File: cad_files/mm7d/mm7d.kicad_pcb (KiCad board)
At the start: 2 copper layers, 56.9 x 67.6 mm, 4 parts

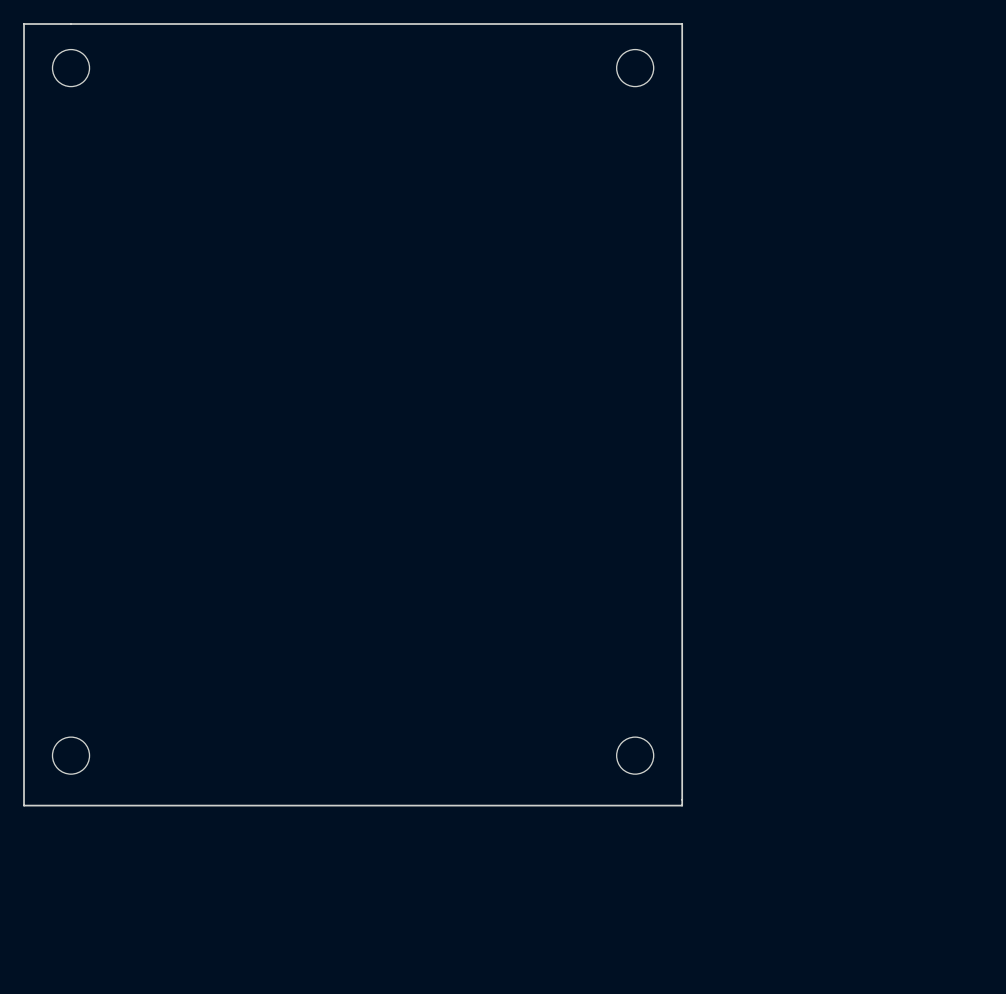
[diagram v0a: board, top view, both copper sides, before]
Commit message: 200705
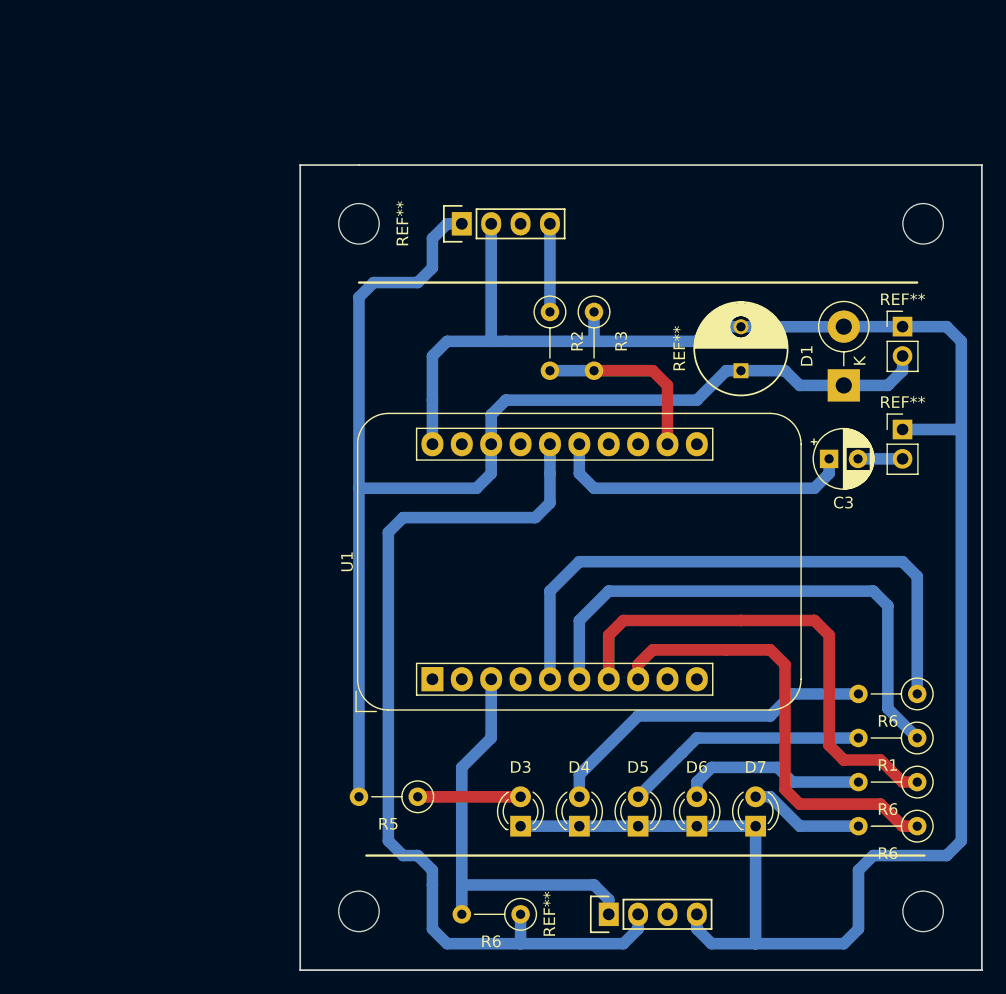
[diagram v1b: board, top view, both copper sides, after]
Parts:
- removed the REF** at (99.1, 114.0)
- removed the REF** at (147.8, 114.0)
- removed the REF** at (147.8, 54.6)
- removed the REF** at (99.1, 54.6)
- added C3: CP_Radial_D5.0mm_P2.50mm, Capacitor_THT:CP_Radial_D5.0mm_P2.50mm, F.Cu at (164.6, 88.4)
- added D1: D_5W_P5.08mm_Vertical_KathodeUp, Diode_THT:D_5W_P5.08mm_Vertical_KathodeUp, F.Cu at (165.9, 82.0)
- added D3: LED_D3.0mm, LED_THT:LED_D3.0mm, F.Cu at (137.9, 120.1)
- added D4: LED_D3.0mm, LED_THT:LED_D3.0mm, F.Cu at (143.0, 120.1)
- added D5: LED_D3.0mm, LED_THT:LED_D3.0mm, F.Cu at (148.1, 120.1)
- added D6: LED_D3.0mm, LED_THT:LED_D3.0mm, F.Cu at (153.2, 120.1)
- added D7: LED_D3.0mm, LED_THT:LED_D3.0mm, F.Cu at (158.2, 120.1)
- added R1: R_Axial_DIN0207_L6.3mm_D2.5mm_P5.08mm_Vertical, Resistor_THT:R_Axial_DIN0207_L6.3mm_D2.5mm_P5.08mm_Vertical, F.Cu at (172.2, 112.5)
- added R2: R_Axial_DIN0207_L6.3mm_D2.5mm_P5.08mm_Vertical, Resistor_THT:R_Axial_DIN0207_L6.3mm_D2.5mm_P5.08mm_Vertical, F.Cu at (140.5, 75.7)
- added R3: R_Axial_DIN0207_L6.3mm_D2.5mm_P5.08mm_Vertical, Resistor_THT:R_Axial_DIN0207_L6.3mm_D2.5mm_P5.08mm_Vertical, F.Cu at (144.3, 75.7)
- added R5: R_Axial_DIN0207_L6.3mm_D2.5mm_P5.08mm_Vertical, Resistor_THT:R_Axial_DIN0207_L6.3mm_D2.5mm_P5.08mm_Vertical, F.Cu at (129.0, 117.6)
- added R6: R_Axial_DIN0207_L6.3mm_D2.5mm_P5.08mm_Vertical, Resistor_THT:R_Axial_DIN0207_L6.3mm_D2.5mm_P5.08mm_Vertical, F.Cu at (137.9, 127.8)
- added R6: R_Axial_DIN0207_L6.3mm_D2.5mm_P5.08mm_Vertical, Resistor_THT:R_Axial_DIN0207_L6.3mm_D2.5mm_P5.08mm_Vertical, F.Cu at (172.2, 120.1)
- added R6: R_Axial_DIN0207_L6.3mm_D2.5mm_P5.08mm_Vertical, Resistor_THT:R_Axial_DIN0207_L6.3mm_D2.5mm_P5.08mm_Vertical, F.Cu at (172.2, 116.3)
- added R6: R_Axial_DIN0207_L6.3mm_D2.5mm_P5.08mm_Vertical, Resistor_THT:R_Axial_DIN0207_L6.3mm_D2.5mm_P5.08mm_Vertical, F.Cu at (172.2, 108.7)
- added REF**: PinHeader_1x02_P2.54mm_Vertical, Connector_PinHeader_2.54mm:PinHeader_1x02_P2.54mm_Vertical, F.Cu at (170.9, 77.0)
- added REF**: MountingHole_3.5mm, MountingHole:MountingHole_3.5mm, F.Cu at (172.7, 68.1)
- added REF**: MountingHole_3.5mm, MountingHole:MountingHole_3.5mm, F.Cu at (172.7, 127.5)
- added REF**: MountingHole_3.5mm, MountingHole:MountingHole_3.5mm, F.Cu at (124.0, 127.5)
- added REF**: MountingHole_3.5mm, MountingHole:MountingHole_3.5mm, F.Cu at (124.0, 68.1)
- added REF**: PinHeader_1x02_P2.54mm_Vertical, Connector_PinHeader_2.54mm:PinHeader_1x02_P2.54mm_Vertical, F.Cu at (170.9, 85.9)
- added REF**: Pin_Header_Straight_1x04, Pin_Headers:Pin_Header_Straight_1x04, F.Cu at (145.5, 127.8)
- added REF**: Pin_Header_Straight_1x04, Pin_Headers:Pin_Header_Straight_1x04, F.Cu at (132.8, 68.1)
- added REF**: C_Radial_D8_L13_P3.8, Capacitors_THT:C_Radial_D8_L13_P3.8, F.Cu at (157.0, 80.8)
- added U1: Adafruit_HUZZAH_ESP8266_breakout, Module:Adafruit_HUZZAH_ESP8266_breakout, F.Cu at (130.3, 107.4)
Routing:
- net (no net): track 0.00 -> 723.0 mm
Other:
- board size 56.9 x 67.6 mm -> 58.9 x 69.6 mm

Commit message: 200705
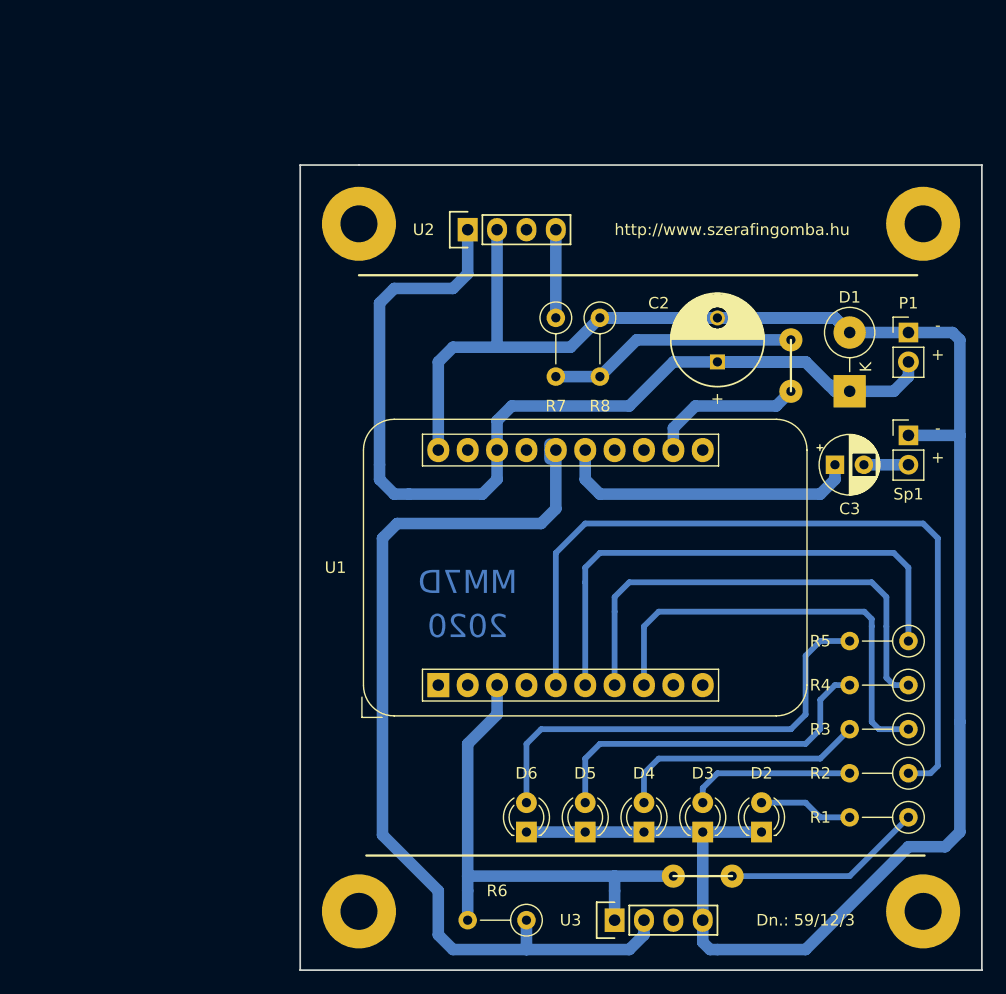
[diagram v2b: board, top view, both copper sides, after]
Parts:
- removed the REF** at (172.7, 68.1)
- removed the REF** at (172.7, 127.5)
- removed the REF** at (124.0, 127.5)
- removed the REF** at (124.0, 68.1)
- added REF**: SolderWirePad_single_0-8mmDrill, Wire_Pads:SolderWirePad_single_0-8mmDrill, F.Cu at (161.3, 82.5)
- added REF**: SolderWirePad_single_0-8mmDrill, Wire_Pads:SolderWirePad_single_0-8mmDrill, F.Cu at (161.3, 78.1)
- added REF**: SolderWirePad_single_0-8mmDrill, Wire_Pads:SolderWirePad_single_0-8mmDrill, F.Cu at (156.2, 124.5)
- added REF**: SolderWirePad_single_0-8mmDrill, Wire_Pads:SolderWirePad_single_0-8mmDrill, F.Cu at (151.1, 124.5)
- added REF**: MountingHole_3.2mm_M3_Pad, Mounting_Holes:MountingHole_3.2mm_M3_Pad, F.Cu at (124.0, 68.1)
- added REF**: MountingHole_3.2mm_M3_Pad, Mounting_Holes:MountingHole_3.2mm_M3_Pad, F.Cu at (172.7, 68.1)
- added REF**: MountingHole_3.2mm_M3_Pad, Mounting_Holes:MountingHole_3.2mm_M3_Pad, F.Cu at (172.7, 127.5)
- added REF**: MountingHole_3.2mm_M3_Pad, Mounting_Holes:MountingHole_3.2mm_M3_Pad, F.Cu at (124.0, 127.5)
- moved R5 44.5 mm to (171.4, 104.1)
- moved C2 2.17 mm to (154.9, 80.0)
- moved R1 1.08 mm to (171.4, 119.4)
- moved R2 1.08 mm to (171.4, 115.6)
- moved R3 1.08 mm to (171.4, 111.8)
- moved R4 1.08 mm to (171.4, 108.0)
- moved D2 0.72 mm to (158.8, 120.7)
- moved D4 0.72 mm to (148.6, 120.7)
- moved D6 0.72 mm to (138.4, 120.7)
- moved R6 0.72 mm to (138.4, 128.3)
- moved R7 0.72 mm to (141.0, 76.2)
- moved R8 0.72 mm to (144.8, 76.2)
- moved U1 0.72 mm to (130.8, 108.0)
- moved U3 0.72 mm to (146.1, 128.3)
- moved D1 0.72 mm to (166.4, 82.5)
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- renumbered REF** to C2, D7 to D2, D6 to D3, D5 to D4, D4 to D5, D3 to D6, REF** to P1, R6 to R1, R6 to R2, R1 to R3, R6 to R4, R2 to R7, R3 to R8, REF** to Sp1, REF** to U2, REF** to U3
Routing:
- net (no net): track 723.0 -> 809.2 mm
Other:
- board text added: "+"
- board text added: "-"
- board text added: "2020"
- board text added: "Dn.: 59/12/3"
- board text added: "MM7D"
- board text added: "http://www.szerafingomba.hu"

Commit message: 200706
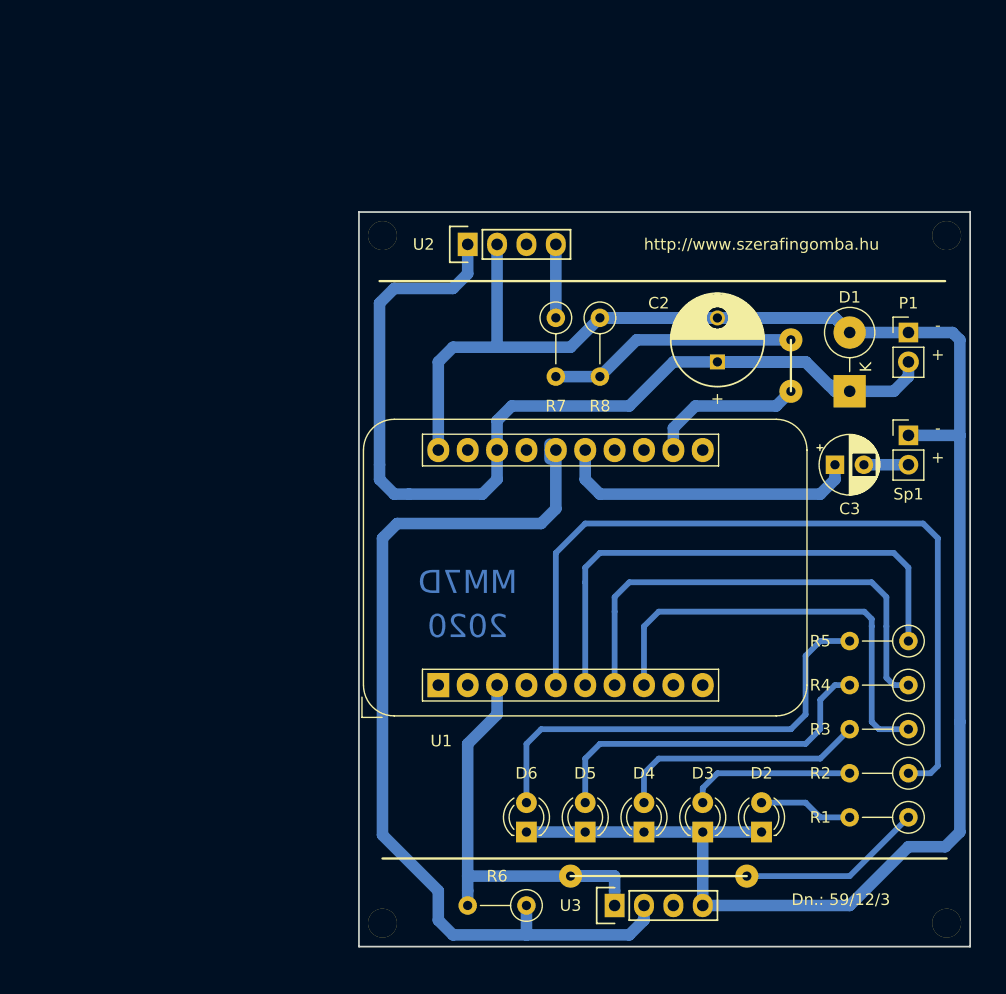
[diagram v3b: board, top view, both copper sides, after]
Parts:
- removed the REF** at (124.0, 68.1)
- removed the REF** at (172.7, 68.1)
- removed the REF** at (172.7, 127.5)
- removed the REF** at (124.0, 127.5)
- added REF**: MountingHole_2.5mm, mm7d:MyMountingHole_2.5mm, F.Cu at (126.0, 69.1)
- added REF**: MountingHole_2.5mm, mm7d:MyMountingHole_2.5mm, F.Cu at (174.8, 69.1)
- added REF**: MountingHole_2.5mm, mm7d:MyMountingHole_2.5mm, F.Cu at (174.8, 128.5)
- added REF**: MountingHole_2.5mm, mm7d:MyMountingHole_2.5mm, F.Cu at (126.0, 128.5)
- moved REF** 8.89 mm to (142.2, 124.5)
- moved R6 1.27 mm to (138.4, 127.0)
- moved U3 1.27 mm to (146.1, 127.0)
- moved U2 1.27 mm to (133.3, 69.8)
- moved REF** 1.27 mm to (157.5, 124.5)
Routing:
- net (no net): track 809.2 -> 794.1 mm
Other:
- board size 58.9 x 69.6 mm -> 52.8 x 63.5 mm

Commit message: 200714
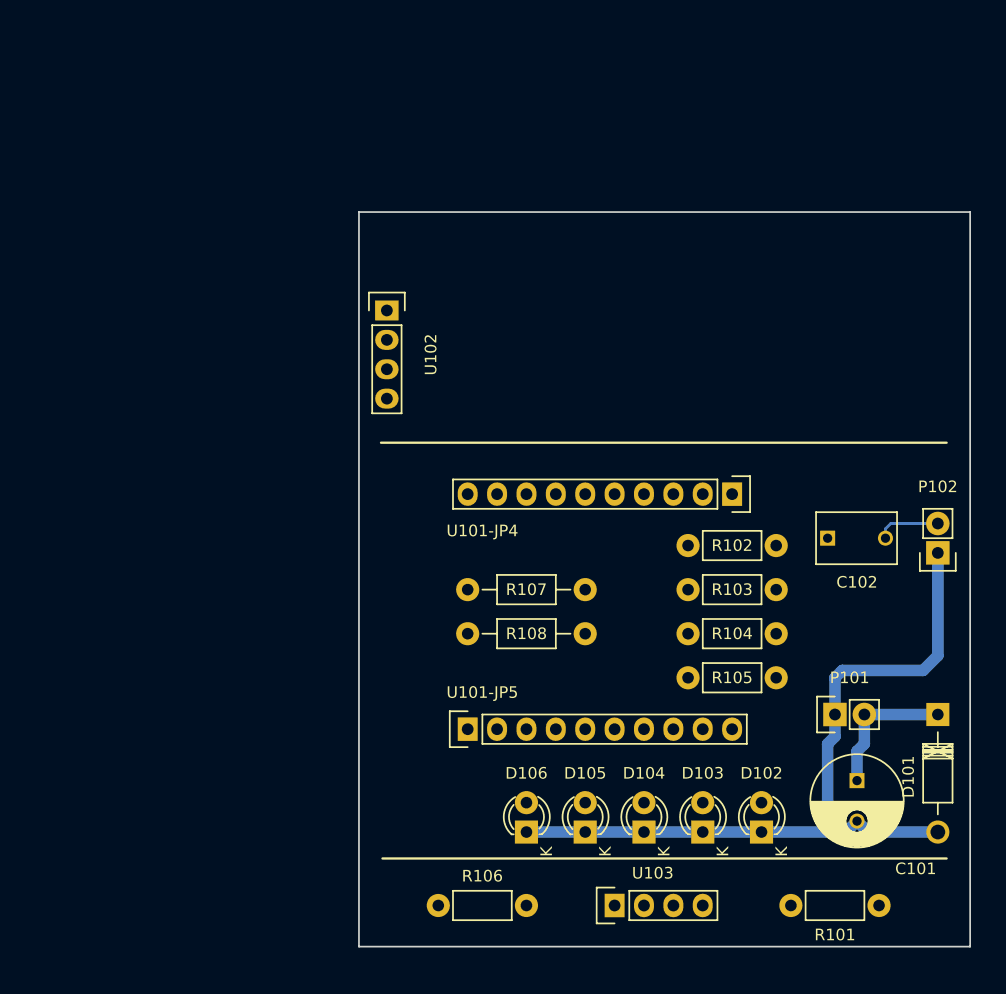
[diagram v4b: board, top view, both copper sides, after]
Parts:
- removed C2: C_Radial_D8_L13_P3.8, Capacitors_THT:C_Radial_D8_L13_P3.8
- removed C3: CP_Radial_D5.0mm_P2.50mm, Capacitor_THT:CP_Radial_D5.0mm_P2.50mm
- removed D1: D_5W_P5.08mm_Vertical_KathodeUp, Diode_THT:D_5W_P5.08mm_Vertical_KathodeUp
- removed P1, Sp1: PinHeader_1x02_P2.54mm_Vertical, Connector_PinHeader_2.54mm:PinHeader_1x02_P2.54mm_Vertical
- removed R1, R2, R3, R4, R5, R6, R7, R8: R_Axial_DIN0207_L6.3mm_D2.5mm_P5.08mm_Vertical, Resistor_THT:R_Axial_DIN0207_L6.3mm_D2.5mm_P5.08mm_Vertical
- removed REF** (x4): SolderWirePad_single_0-8mmDrill, Wire_Pads:SolderWirePad_single_0-8mmDrill
- removed REF** (x4): MountingHole_2.5mm, mm7d:MyMountingHole_2.5mm
- removed U1: Adafruit_HUZZAH_ESP8266_breakout, Module:Adafruit_HUZZAH_ESP8266_breakout
- removed U2, U3: Pin_Header_Straight_1x04, Pin_Headers:Pin_Header_Straight_1x04
- added C101: 470u, Capacitors_THT:C_Radial_D8_L11.5_P3.5, F.Cu at (167.0, 116.2)
- added C102: 2.2u, Capacitors_THT:C_Rect_L7_W4.5_P5, F.Cu at (164.5, 95.2)
- added D101: 1N4001, Diodes_THT:Diode_DO-41_SOD81_Horizontal_RM10, F.Cu at (174.0, 110.5)
- added P101: CONN_01X02, Socket_Strips:Socket_Strip_Straight_1x02, F.Cu at (165.1, 110.5)
- added P102: CONN_01X02, Socket_Strips:Socket_Strip_Straight_1x02, F.Cu at (174.0, 96.5)
- added R101: 470, Resistors_THT:Resistor_Horizontal_RM7mm, F.Cu at (168.9, 127.0)
- added R102: 470, Resistors_THT:Resistor_Horizontal_RM7mm, F.Cu at (152.4, 95.9)
- added R103: 470, Resistors_THT:Resistor_Horizontal_RM7mm, F.Cu at (152.4, 99.7)
- added R104: 470, Resistors_THT:Resistor_Horizontal_RM7mm, F.Cu at (152.4, 103.5)
- added R105: 470, Resistors_THT:Resistor_Horizontal_RM7mm, F.Cu at (152.4, 107.3)
- added R106: 4.7k, Resistors_THT:Resistor_Horizontal_RM7mm, F.Cu at (130.8, 127.0)
- added R107: 39k, Resistors_THT:Resistor_Horizontal_RM10mm, F.Cu at (133.3, 99.7)
- added R108: 9.1k, Resistors_THT:Resistor_Horizontal_RM10mm, F.Cu at (133.3, 103.5)
- added U101-JP4: CONN_01X10, Socket_Strips:Socket_Strip_Straight_1x10, F.Cu at (156.2, 91.4)
- added U101-JP5: CONN_01X10, Socket_Strips:Socket_Strip_Straight_1x10, F.Cu at (133.3, 111.8)
- added U102: MQ-135M, Socket_Strips:Socket_Strip_Straight_1x04, F.Cu at (126.4, 75.6)
- added U103: DHT11, Socket_Strips:Socket_Strip_Straight_1x04, F.Cu at (146.1, 127.0)
- D102: renamed from D2; value LED_D3.0mm -> white; footprint LED_THT:LED_D3.0mm -> LEDs:LED-3MM
- D103: renamed from D3; value LED_D3.0mm -> blue; footprint LED_THT:LED_D3.0mm -> LEDs:LED-3MM
- D104: renamed from D4; value LED_D3.0mm -> green; footprint LED_THT:LED_D3.0mm -> LEDs:LED-3MM
- D105: renamed from D5; value LED_D3.0mm -> yellow; footprint LED_THT:LED_D3.0mm -> LEDs:LED-3MM
- D106: renamed from D6; value LED_D3.0mm -> red; footprint LED_THT:LED_D3.0mm -> LEDs:LED-3MM
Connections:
- D102 pad 1: (no net) -> GND
- D102 pad 2: (no net) -> Net-(D102-Pad2)
- D103 pad 1: (no net) -> GND
- D103 pad 2: (no net) -> Net-(D103-Pad2)
- D104 pad 1: (no net) -> GND
- D104 pad 2: (no net) -> Net-(D104-Pad2)
- D105 pad 1: (no net) -> GND
- D105 pad 2: (no net) -> Net-(D105-Pad2)
- D106 pad 1: (no net) -> GND
- D106 pad 2: (no net) -> Net-(D106-Pad2)
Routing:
- net (no net): track 794.1 -> 0.00 mm
- net GND: track 0.00 -> 68.5 mm
- net +5V: track 0.00 -> 12.3 mm
- net Net-(C102-Pad2): track 0.00 -> 5.52 mm
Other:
- board text removed: "+"
- board text removed: "-"
- board text removed: "2020"
- board text removed: "Dn.: 59/12/3"
- board text removed: "MM7D"
- board text removed: "http://www.szerafingomba.hu"
